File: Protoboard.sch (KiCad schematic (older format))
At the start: 11 parts, among them P1 CONN_01X08, P2 CONN_01X04, P3 CONN_01X05, P4 CONN_01X04, P5 CONN_02X05, P6 CONN_01X10

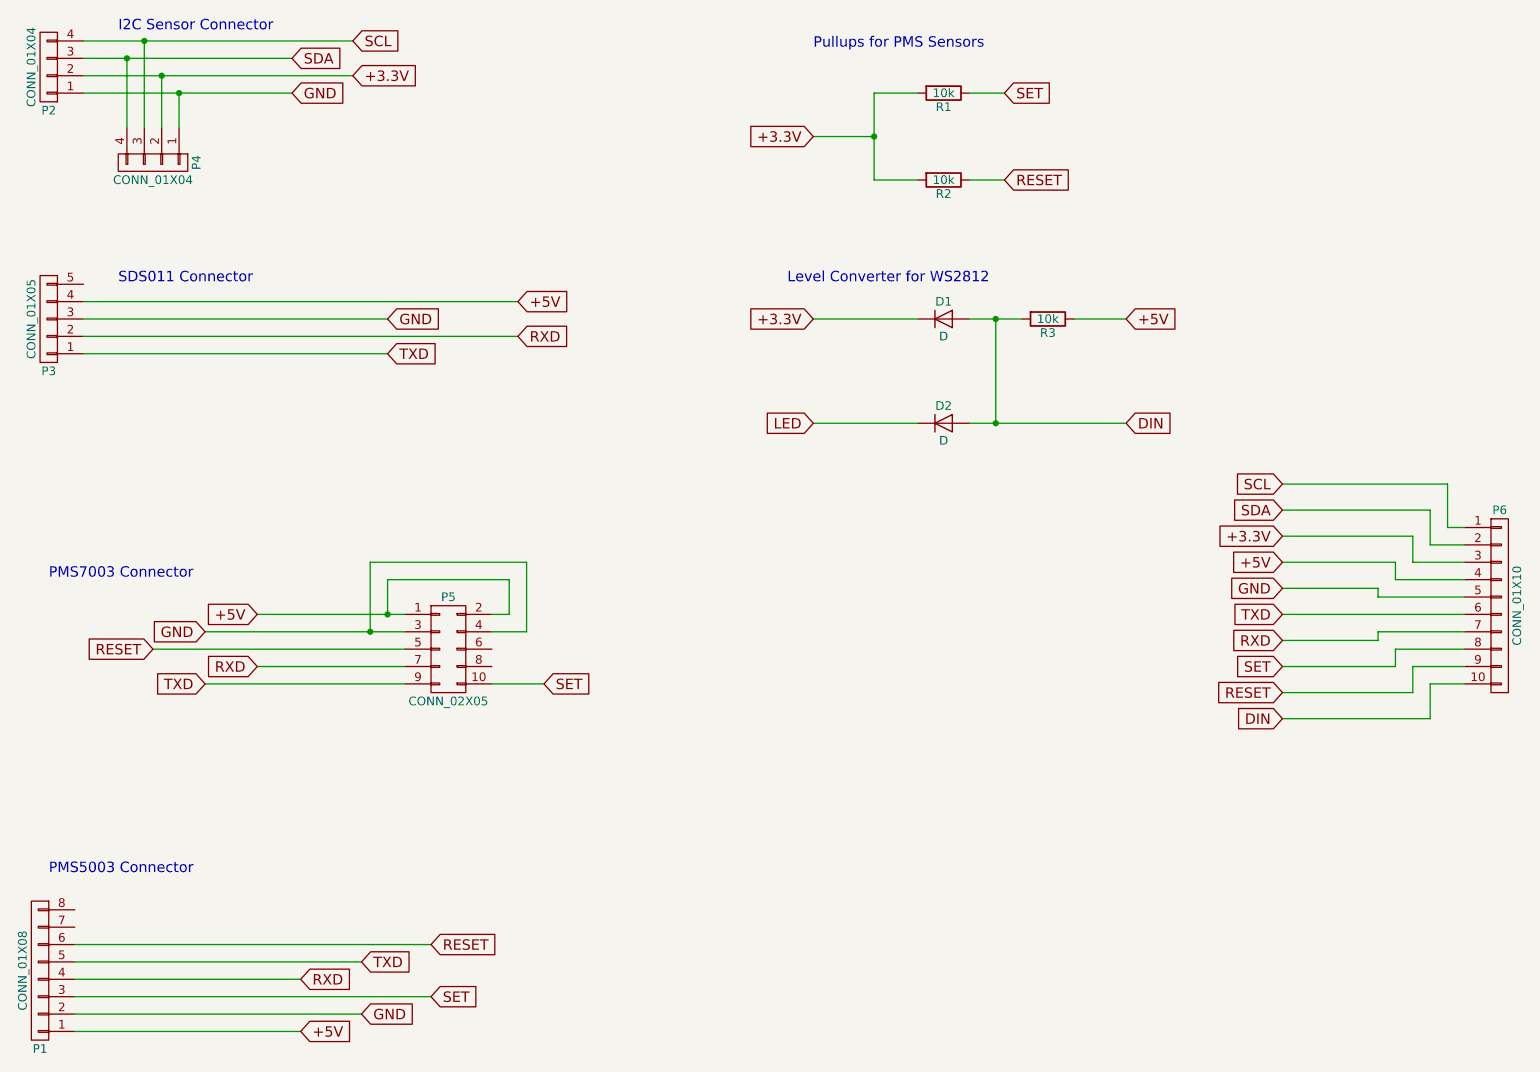
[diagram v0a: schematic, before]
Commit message: Routing done.
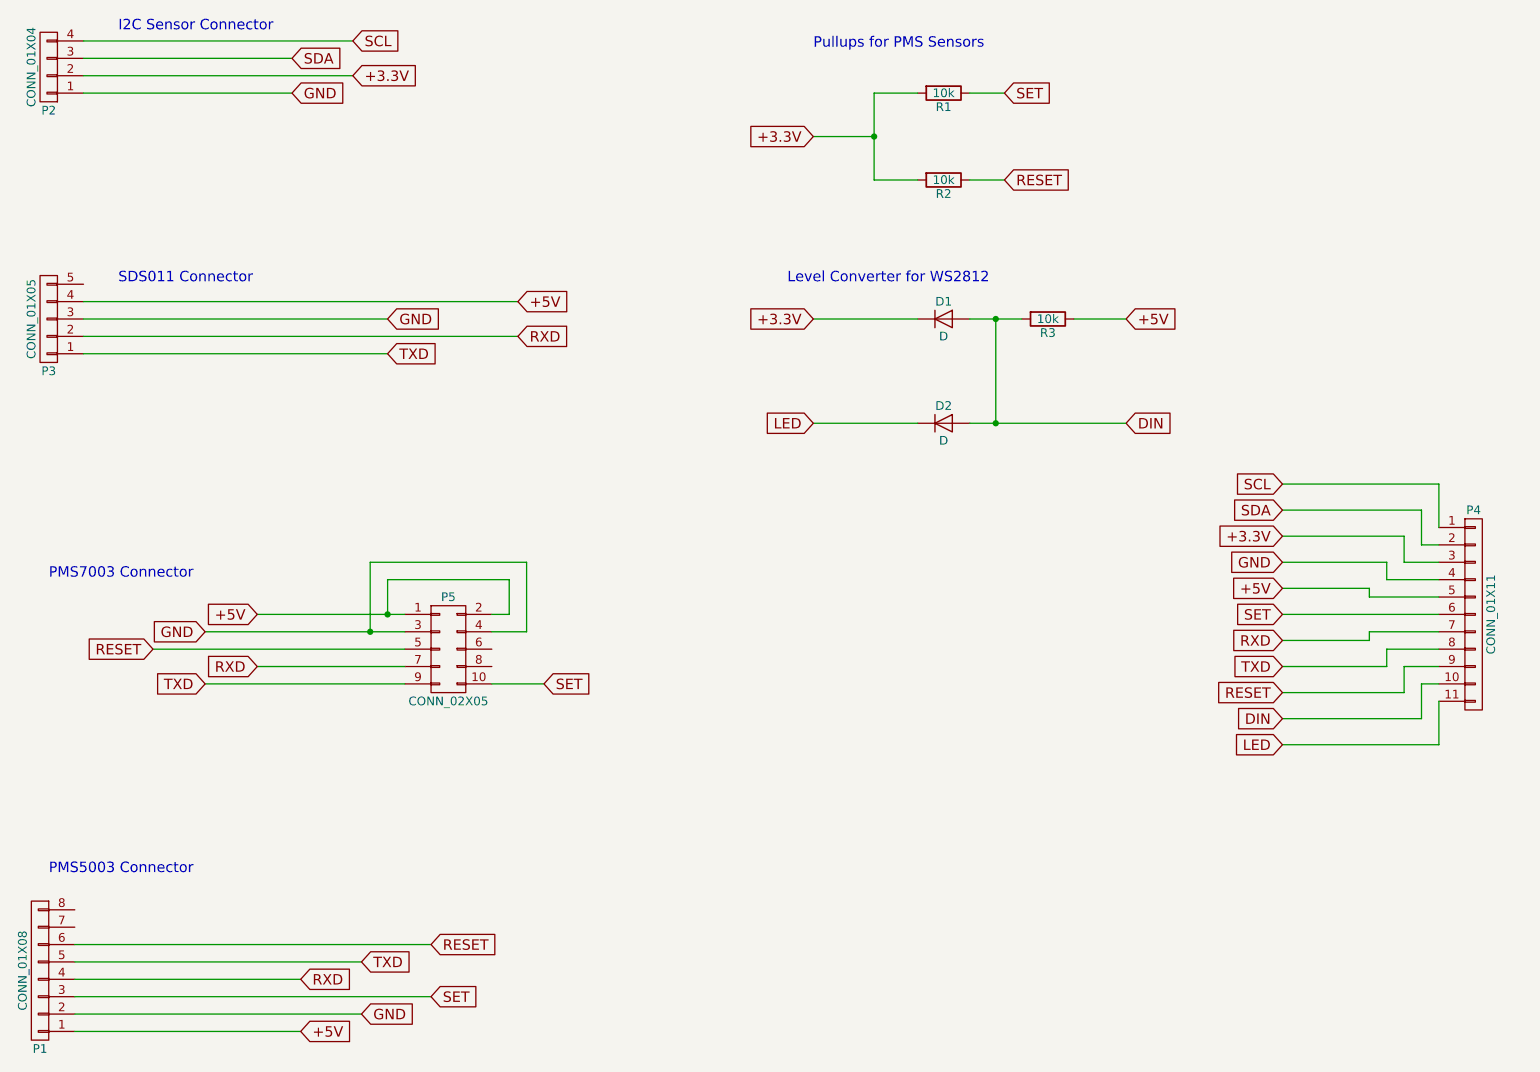
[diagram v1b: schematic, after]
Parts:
- removed P4: CONN_01X04, Pin_Headers:Pin_Header_Straight_1x04, symbol CONN_01X04
- removed P6: CONN_01X10, Pin_Headers:Pin_Header_Straight_1x10, symbol CONN_01X10
- added P4: CONN_01X11, Pin_Headers:Pin_Header_Straight_1x11, symbol CONN_01X11
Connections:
- net +3.3V: now also P4.3 (P3)
- net +5V: now also P4.5 (P5)
- net DIN: now also P4.10 (P10)
- net GND: now also P4.4 (P4)
- net LED: now also P4.11 (P11)
- net RESET: now also P4.9 (P9)
- net RXD: now also P4.7 (P7)
- net SCL: now also P4.1 (P1)
- net SDA: now also P4.2 (P2)
- net SET: now also P4.6 (P6)
- net TXD: now also P4.8 (P8)
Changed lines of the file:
@@
 	-1   0    0    1
-$EndComp
-$Comp
-L CONN_01X04 P4
-U 1 1 58C4517D
-P 1600 1600
-F 0 "P4" H 1600 1850 50  0000 C CNN
-F 1 "CONN_01X04" V 1700 1600 50  0000 C CNN
-F 2 "Pin_Headers:Pin_Header_Straight_1x04" H 1600 1600 50  0001 C CNN
-F 3 "" H 1600 1600 50  0000 C CNN
-	1    1600 1600
-	0    1    1    0
 $EndComp
 Text GLabel 2400 1200 2    60   Input ~ 0
@@
 	1200 1200 2400 1200
 Wire Wire Line
-	1750 1400 1750 1200
-Connection ~ 1750 1200
-Wire Wire Line
 	1200 1100 2750 1100
 Wire Wire Line
-	1650 1400 1650 1100
-Connection ~ 1650 1100
-Wire Wire Line
-	2400 1000 1200 1000
-Wire Wire Line
-	1450 1400 1450 1000
-Connection ~ 1450 1000
-Wire Wire Line
 	2750 900  1200 900
-Wire Wire Line
-	1550 1400 1550 900
-Connection ~ 1550 900
 Text Notes 1400 850  0    60   ~ 0
 I2C Sensor Connector\n
@@
 Text GLabel 8100 3750 0    60   Input ~ 0
 +3.3V
+Text GLabel 8100 4050 0    60   Input ~ 0
++5V
 Text GLabel 8100 3900 0    60   Input ~ 0
-+5V
-Text GLabel 8100 4050 0    60   Input ~ 0
-GND
-Text GLabel 8100 4200 0    60   Input ~ 0
+GND
+Text GLabel 8100 4500 0    60   Input ~ 0
 TXD
 Text GLabel 8100 4350 0    60   Input ~ 0
 RXD
-Text GLabel 8100 4500 0    60   Input ~ 0
+Text GLabel 8100 4200 0    60   Input ~ 0
 SET
 Text GLabel 8100 4650 0    60   Input ~ 0
@@
 Text GLabel 8100 4800 0    60   Input ~ 0
 DIN
-$Comp
-L CONN_01X10 P6
-U 1 1 58C59B8A
-P 9350 4150
-F 0 "P6" H 9350 4700 50  0000 C CNN
-F 1 "CONN_01X10" V 9450 4150 50  0000 C CNN
-F 2 "Pin_Headers:Pin_Header_Straight_1x10" H 9350 4150 50  0001 C CNN
-F 3 "" H 9350 4150 50  0000 C CNN
-	1    9350 4150
+Text GLabel 8100 4950 0    60   Input ~ 0
+LED
+Wire Wire Line
+	2400 1000 1200 1000
+$Comp
+L CONN_01X11 P4
+U 1 1 58C5C7BE
+P 9200 4200
+F 0 "P4" H 9200 4800 50  0000 C CNN
+F 1 "CONN_01X11" V 9300 4200 50  0000 C CNN
+F 2 "Pin_Headers:Pin_Header_Straight_1x11" H 9200 4200 50  0001 C CNN
+F 3 "" H 9200 4200 50  0000 C CNN
+	1    9200 4200
 	1    0    0    -1
 $EndComp
 Wire Wire Line
-	9150 3700 9050 3700
-Wire Wire Line
-	9050 3700 9050 3450
-Wire Wire Line
-	9050 3450 8100 3450
-Wire Wire Line
-	9150 3800 8950 3800
-Wire Wire Line
-	8950 3800 8950 3600
-Wire Wire Line
-	8950 3600 8100 3600
-Wire Wire Line
-	9150 3900 8850 3900
-Wire Wire Line
-	8850 3900 8850 3750
-Wire Wire Line
-	8850 3750 8100 3750
-Wire Wire Line
-	9150 4000 8750 4000
-Wire Wire Line
-	8750 4000 8750 3900
-Wire Wire Line
-	8750 3900 8100 3900
-Wire Wire Line
-	9150 4100 8650 4100
-Wire Wire Line
-	8650 4100 8650 4050
-Wire Wire Line
-	8650 4050 8100 4050
-Wire Wire Line
-	9150 4200 8100 4200
-Wire Wire Line
-	9150 4300 8650 4300
-Wire Wire Line
-	8650 4300 8650 4350
-Wire Wire Line
-	8650 4350 8100 4350
-Wire Wire Line
-	9150 4400 8750 4400
-Wire Wire Line
-	8750 4400 8750 4500
-Wire Wire Line
-	8750 4500 8100 4500
-Wire Wire Line
-	9150 4500 8850 4500
-Wire Wire Line
-	8850 4500 8850 4650
-Wire Wire Line
-	8850 4650 8100 4650
-Wire Wire Line
-	9150 4600 8950 4600
-Wire Wire Line
-	8950 4600 8950 4800
-Wire Wire Line
-	8950 4800 8100 4800
+	8100 3450 9000 3450
+Wire Wire Line
+	9000 3450 9000 3700
+Wire Wire Line
+	9000 3800 8900 3800
+Wire Wire Line
+	8900 3800 8900 3600
+Wire Wire Line
+	8900 3600 8100 3600
+Wire Wire Line
+	9000 3900 8800 3900
+Wire Wire Line
+	8800 3900 8800 3750
+Wire Wire Line
+	8800 3750 8100 3750
+Wire Wire Line
+	8100 3900 8700 3900
+Wire Wire Line
+	8700 3900 8700 4000
+Wire Wire Line
+	8700 4000 9000 4000
+Wire Wire Line
+	9000 4100 8600 4100
+Wire Wire Line
+	8600 4100 8600 4050
+Wire Wire Line
+	8600 4050 8100 4050
+Wire Wire Line
+	9000 4200 8100 4200
+Wire Wire Line
+	9000 4300 8600 4300
+Wire Wire Line
+	8600 4300 8600 4350
+Wire Wire Line
+	8600 4350 8100 4350
+Wire Wire Line
+	8100 4500 8700 4500
+Wire Wire Line
+	8700 4500 8700 4400
+Wire Wire Line
+	8700 4400 9000 4400
+Wire Wire Line
+	9000 4500 8800 4500
+Wire Wire Line
+	8800 4500 8800 4650
+Wire Wire Line
+	8800 4650 8100 4650
+Wire Wire Line
+	9000 4600 8900 4600
+Wire Wire Line
+	8900 4600 8900 4800
+Wire Wire Line
+	8900 4800 8100 4800
+Wire Wire Line
+	9000 4700 9000 4950
+Wire Wire Line
+	9000 4950 8100 4950
 $EndSCHEMATC
